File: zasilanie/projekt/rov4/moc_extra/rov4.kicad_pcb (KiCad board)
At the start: 2 copper layers, 124.5 x 68.6 mm, 18 parts, among them J43 Torpedy_serwo_7v, J44 Extra, J45 Extra, J46 Manip_serwo, J47 Extra, J48 Extra, J53 HP_IN, J60 HP_OUT, U4 lm2596, U5 lm2596

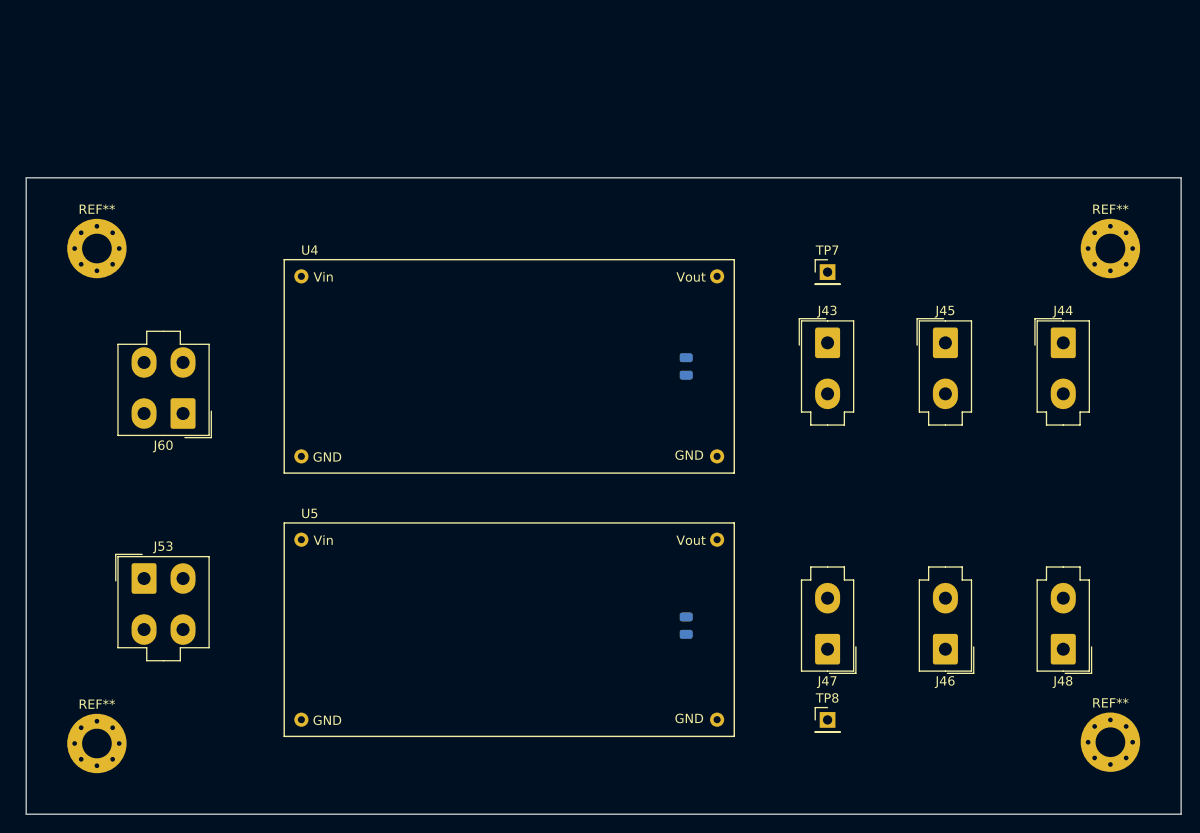
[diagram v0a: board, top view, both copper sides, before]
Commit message: sprzątanie
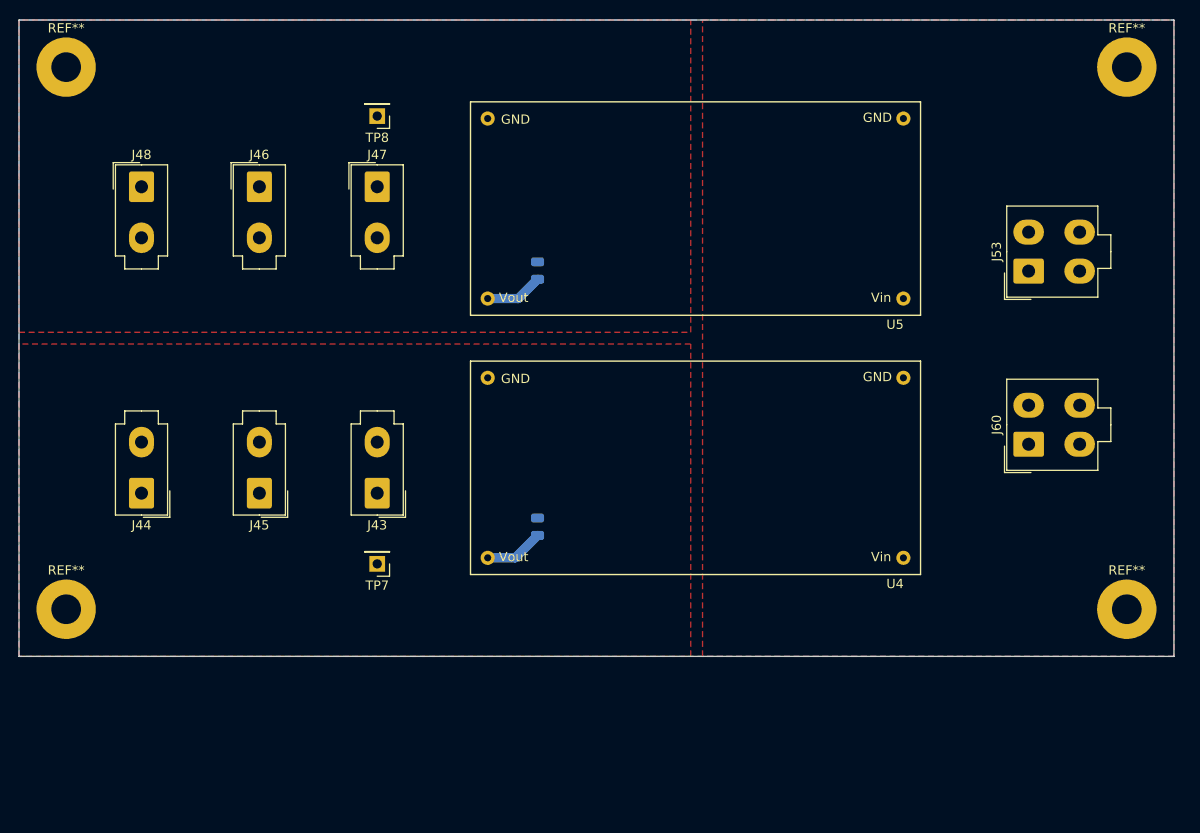
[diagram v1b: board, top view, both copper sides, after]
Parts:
- removed the REF** at (152.3, 101.8)
- removed the REF** at (152.3, 48.6)
- removed the REF** at (43.0, 102.0)
- removed the REF** at (43.0, 48.6)
- added REF**: MountingHole_3.2mm_M3_Pad, MountingHole:MountingHole_3.2mm_M3_Pad, F.Cu at (154.0, 29.1)
- added REF**: MountingHole_3.2mm_M3_Pad, MountingHole:MountingHole_3.2mm_M3_Pad, F.Cu at (154.0, 87.5)
- added REF**: MountingHole_3.2mm_M3_Pad, MountingHole:MountingHole_3.2mm_M3_Pad, F.Cu at (39.7, 87.5)
- added REF**: MountingHole_3.2mm_M3_Pad, MountingHole:MountingHole_3.2mm_M3_Pad, F.Cu at (39.7, 29.1)
- moved J48 111.1 mm to (47.9, 42.0), turned to 0 degrees
- moved J53 100.9 mm to (143.5, 51.1), turned to 90 degrees
- moved J44 100.6 mm to (47.9, 75.0), turned to 180 degrees
- moved J60 91.2 mm to (143.5, 69.7), turned to 90 degrees
- moved J46 89.2 mm to (60.6, 42.0), turned to 0 degrees
- moved TP8 81.2 mm to (73.3, 34.4), turned to 180 degrees
- moved J45 75.7 mm to (60.6, 75.0), turned to 180 degrees
- moved J47 69.6 mm to (73.3, 42.0), turned to 0 degrees
- moved TP7 57.8 mm to (73.3, 82.6), turned to 180 degrees
- moved J43 51.2 mm to (73.3, 75.0), turned to 180 degrees
- moved U5 49.6 mm to (107.6, 44.3), turned to 180 degrees
- moved C28 41.5 mm to (90.5, 51.0), turned to 90 degrees
- moved C27 23.6 mm to (90.5, 78.6), turned to 90 degrees
- moved U4 22.9 mm to (107.6, 72.3), turned to 180 degrees
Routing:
- net Net-(C27-Pad1): track 0.00 -> 6.37 mm
- net Net-(C28-Pad1): track 0.00 -> 6.24 mm
- added copper zone on F.Cu, net Net-(C27-Pad1)
- added copper zone on B.Cu, net Net-(C27-Pad2)
- added copper zone on F.Cu, net Net-(C28-Pad1)
- added copper zone on F.Cu, net Net-(J53-Pad1)
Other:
- rule via_min_size: 0.4 -> 0.5
